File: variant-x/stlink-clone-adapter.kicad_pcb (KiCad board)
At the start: 2 copper layers, 25.4 x 15 mm, 5 parts, among them J1 Conn_01x04, J2 Conn_01x04, J3 2X5_HDR, J4 Conn_01x04, J5 ARM_10PIN

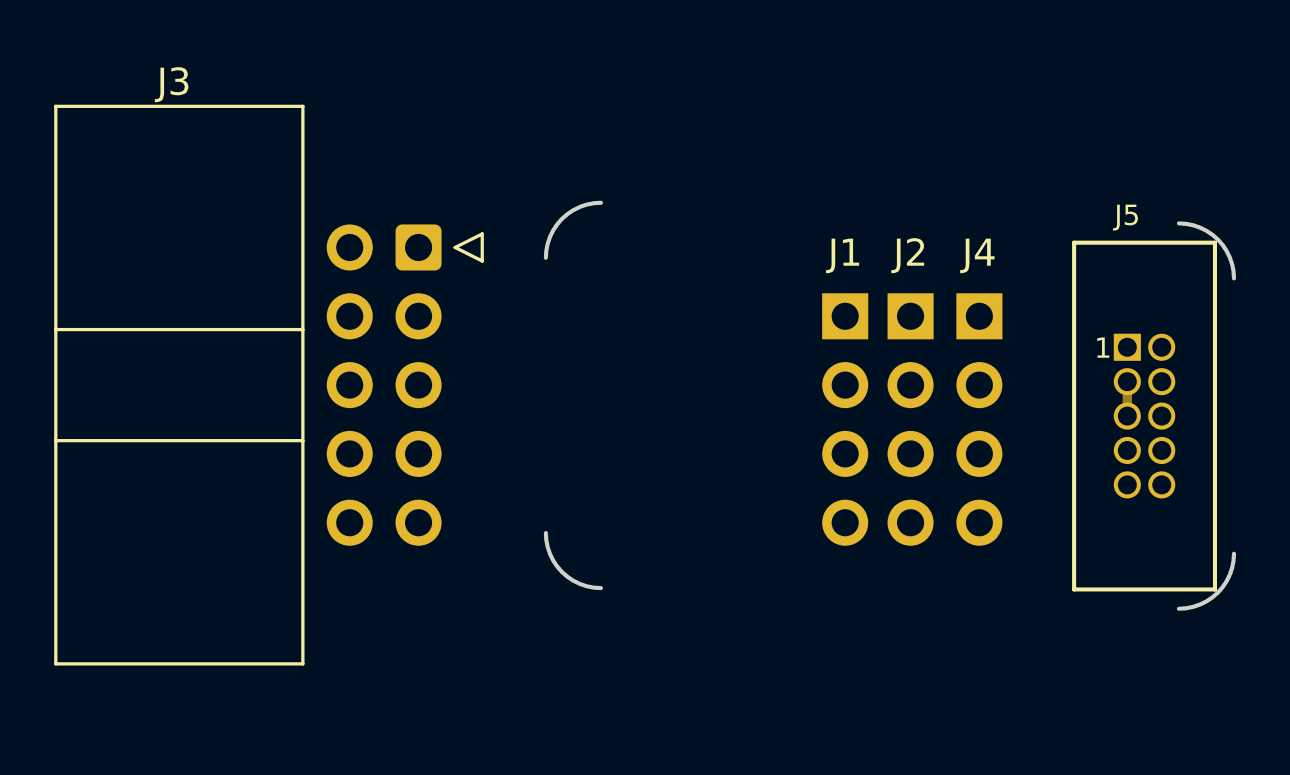
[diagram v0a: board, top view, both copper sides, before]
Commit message: variant-x plot done
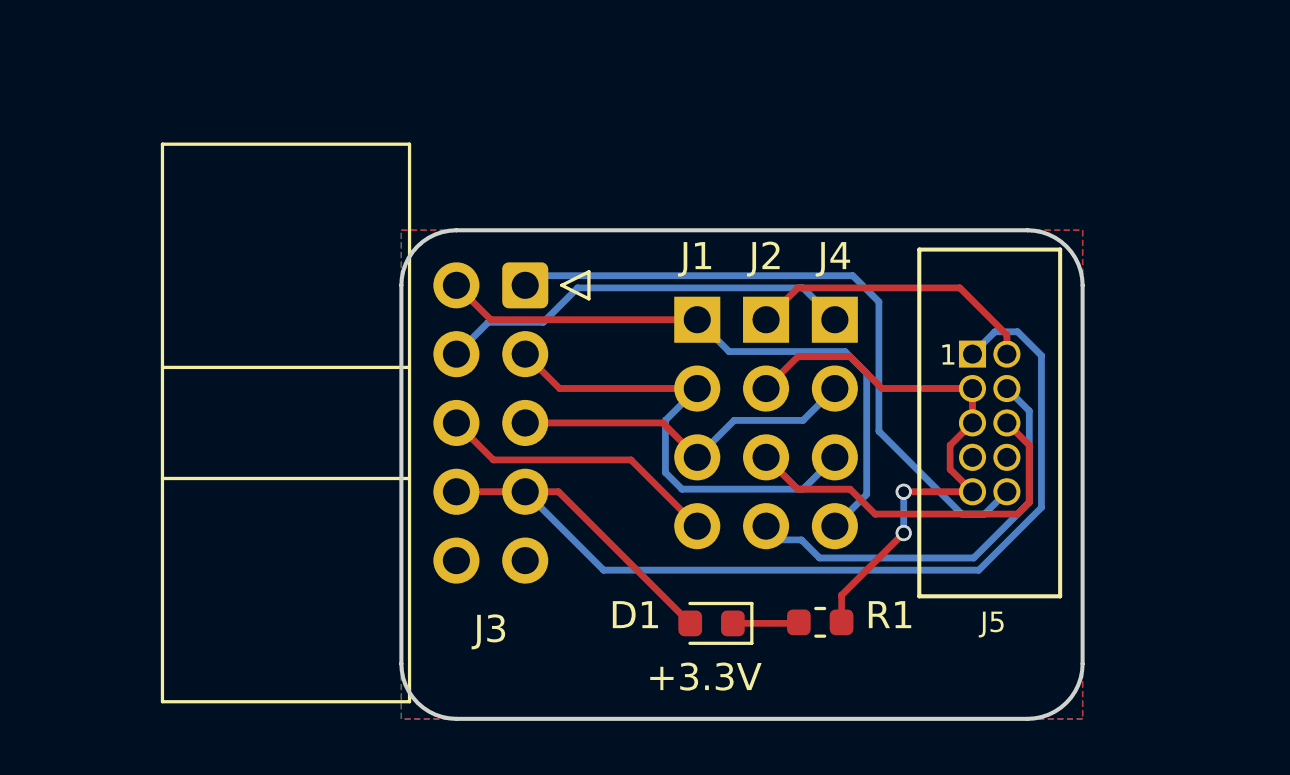
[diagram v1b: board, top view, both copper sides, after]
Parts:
- added D1: LED, LED_SMD:LED_0603_1608Metric, F.Cu at (141.5, 117.9)
- added R1: R, Resistor_SMD:R_0603_1608Metric, F.Cu at (145.5, 117.8)
- added REF**: snowflake, project-lib:snowflake, F.Cu at (143.3, 115.3)
- moved J5 5.72 mm to (151.8, 110.5)
- moved J1 5.46 mm to (141.0, 106.7)
- moved J2 5.34 mm to (143.5, 106.7)
- moved J4 5.34 mm to (146.1, 106.7)
- moved J3 4.18 mm to (119.4, 105.4)
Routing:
- net /3.3V: track 0.00 -> 40.7 mm
- net /RST: track 0.00 -> 24.7 mm
- net /SWDIO|SWCLK: track 0.00 -> 22.6 mm
- net /GND: track 1.27 -> 21.4 mm, vias 0 -> 2
- net /GND|SWIM: track 0.00 -> 17.5 mm
- net /SWCLK: track 0.00 -> 15.6 mm
- net /GND|SWDIO: track 0.00 -> 15.5 mm
- net /SWIM: track 0.00 -> 14.0 mm
- net /SWIM|GND: track 0.00 -> 13.0 mm
- net /SWDIO: track 0.00 -> 10.8 mm
- net /SWCLK|GND: track 0.00 -> 10.5 mm
- net Net-(D1-Pad1): track 0.00 -> 2.45 mm
- added copper zone on F.Cu, net (none)
- added copper zone on B.Cu, net /GND
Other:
- board size 25.4 x 15 mm -> 25.1 x 18 mm
- board text added: "+3.3V"
